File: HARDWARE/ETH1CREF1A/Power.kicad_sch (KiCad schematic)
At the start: 63 parts, among them J601 Conn_02x06_Odd_Even, Q1 IRFR5410, U302 THL15-2415WI, U403 LT8330_S6, U404 LT8330_S6, U406 MC7815CD2TG, U407 MC7915CD2TR4G, U408 TSR1-2450, U408 TSR1-2490, U409 LM1117DTX-3.3/NOPB, U409 LM1117DTX-5/NOPB, U601 MAX5902

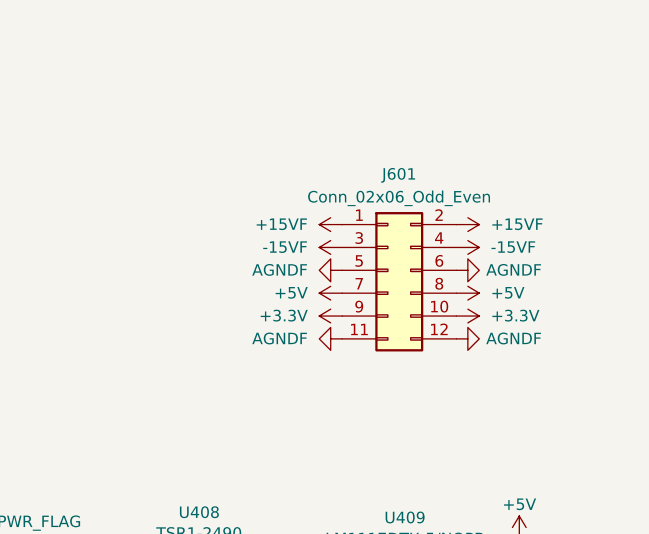
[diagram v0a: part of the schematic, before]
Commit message: Hardware
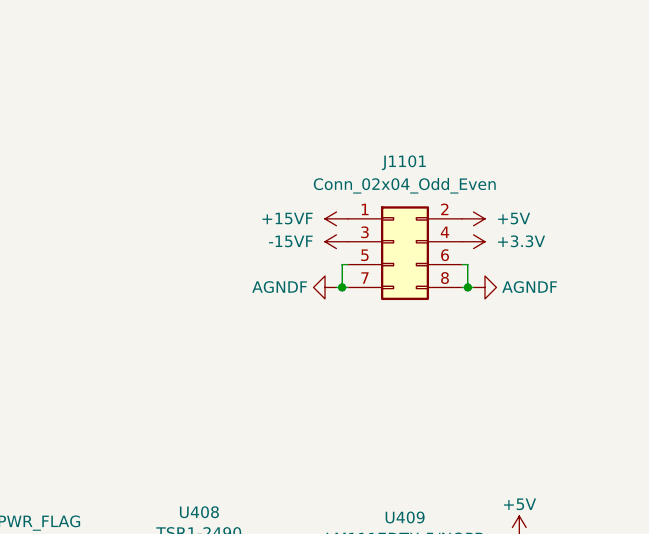
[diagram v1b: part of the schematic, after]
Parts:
- removed J601: Conn_02x06_Odd_Even, Connector_PinHeader_2.54mm:PinHeader_2x06_P2.54mm_Vertical, symbol Connector_Generic:Conn_02x06_Odd_Even
- added J1101: Conn_02x04_Odd_Even, Connector_PinHeader_2.54mm:PinHeader_2x04_P2.54mm_Vertical, symbol Connector_Generic:Conn_02x04_Odd_Even
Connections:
- net +15VF: now also J1101.1 (Pin_1)
- net +3.3V: now also J1101.4 (Pin_4)
- net +5V: now also J1101.2 (Pin_2)
- net -15VF: now also J1101.3 (Pin_3)
- net AGNDF: now also J1101.5 (Pin_5), J1101.6 (Pin_6), J1101.7 (Pin_7), J1101.8 (Pin_8)
